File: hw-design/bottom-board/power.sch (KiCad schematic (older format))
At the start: 13 parts, among them U1 MURATA 5V

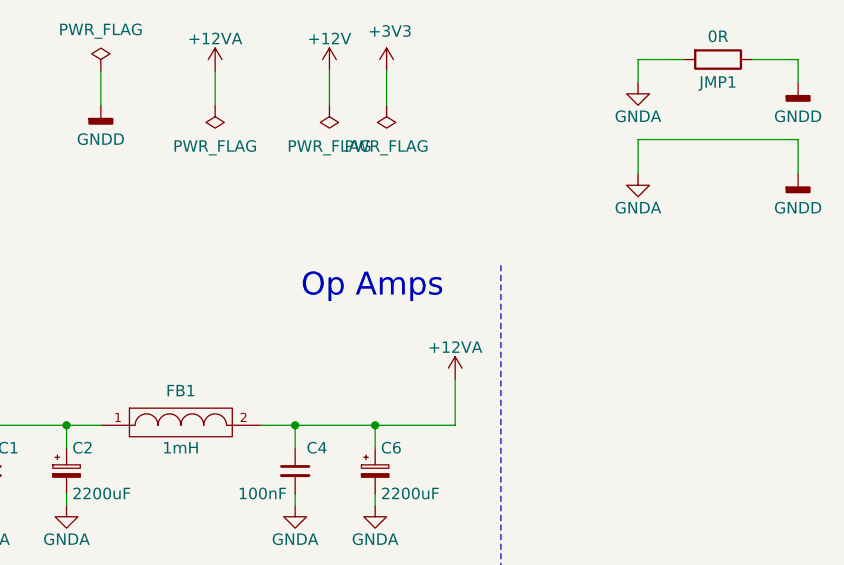
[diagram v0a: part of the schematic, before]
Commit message: added final BOM files
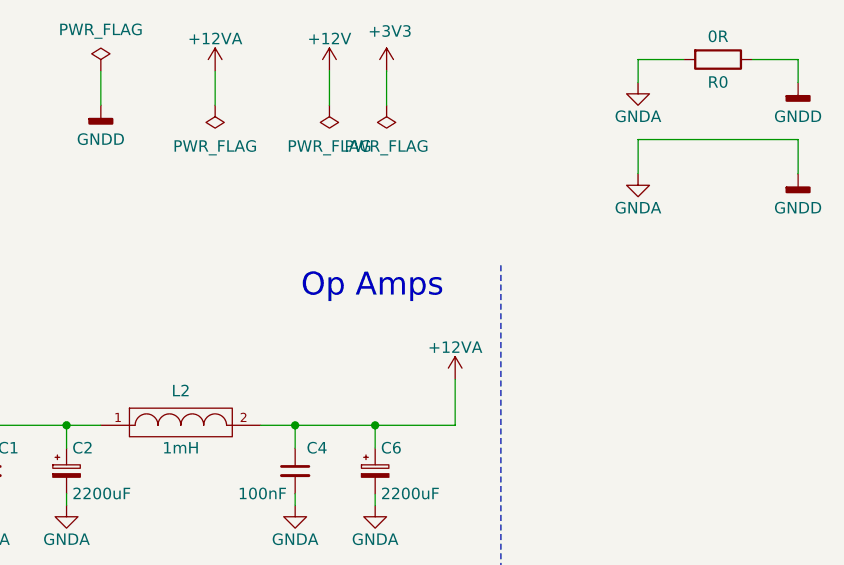
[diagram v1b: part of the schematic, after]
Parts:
- C3, C7: footprint Capacitors_SMD:C_0805 -> Capacitor_SMD:C_0805_2012Metric
- renumbered FB1 to L2, JMP1 to R0
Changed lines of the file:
@@
 $EndComp
 $Comp
-L bottom-board-rescue:FILTER FB1
+L bottom-board-rescue:FILTER L2
 U 1 1 54F8818E
 P 4800 2850
-F 0 "FB1" H 4800 3000 50  0000 C CNN
+F 0 "L2" H 4800 3000 50  0000 C CNN
 F 1 "1mH" H 4800 2750 50  0000 C CNN
 F 2 "Inductors:SELF-WE-PD-XXL" H 4800 2850 60  0001 C CNN
@@
 $EndComp
 $Comp
-L bottom-board-rescue:R JMP1
+L bottom-board-rescue:R R0
 U 1 1 55418B88
 P 7150 1250
-F 0 "JMP1" V 7250 1250 50  0000 C CNN
+F 0 "R0" V 7250 1250 50  0000 C CNN
 F 1 "0R" V 7050 1250 50  0000 C CNN
 F 2 "footprints:Jumper_SMD_THT" V 7080 1250 30  0001 C CNN
@@
 F 0 "C7" H 5900 4950 50  0000 L CNN
 F 1 "10uF" H 5650 4750 50  0000 L CNN
-F 2 "Capacitors_SMD:C_0805" H 5850 4850 60  0001 C CNN
+F 2 "Capacitor_SMD:C_0805_2012Metric" H 5850 4850 60  0001 C CNN
 F 3 "" H 5850 4850 60  0000 C CNN
 F 4 "GRM219R61E106KA12D" H 550 -500 50  0001 C CNN "MPN"
@@
 F 0 "C3" H 4350 4950 50  0000 L CNN
 F 1 "10uF" H 4100 4750 50  0000 L CNN
-F 2 "Capacitors_SMD:C_0805" H 4300 4850 60  0001 C CNN
+F 2 "Capacitor_SMD:C_0805_2012Metric" H 4300 4850 60  0001 C CNN
 F 3 "" H 4300 4850 60  0000 C CNN
 F 4 "GRM219R61E106KA12D" H -1000 -500 50  0001 C CNN "MPN"
